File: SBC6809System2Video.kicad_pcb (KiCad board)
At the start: 4 copper layers, 161.3 x 101.9 mm, 82 parts, among them J1 DIN-9, J10 Conn_01x04, J11 Audio, J12 Conn_01x08, J13 Conn_01x08, J14 Conn_01x08, J15 Conn_01x08, J16 Conn_01x16, J17 Conn_01x08, J18 Conn_01x06, J2 Conn_Coaxial, J3 JTAG, J4 Conn_01x08, J5 Conn_01x16, J6 Conn_01x04, J7 Conn_01x08, J8 Conn_01x06, J9 Conn_01x08, U1 IDT7006L35J, U10 74LS157, U11 74LS157, U12 74LS157, U13 74LS157, U14 74LS157, U15 27C64, U16 74LS157, U2 ATF1504AS, U4 MC68B45, U5 MC68B21, U6 AD725, U7 74HCT393, U8 CD4052B, U9 GAL16V8, Y1 4.433618MHz, Y2 32MHz

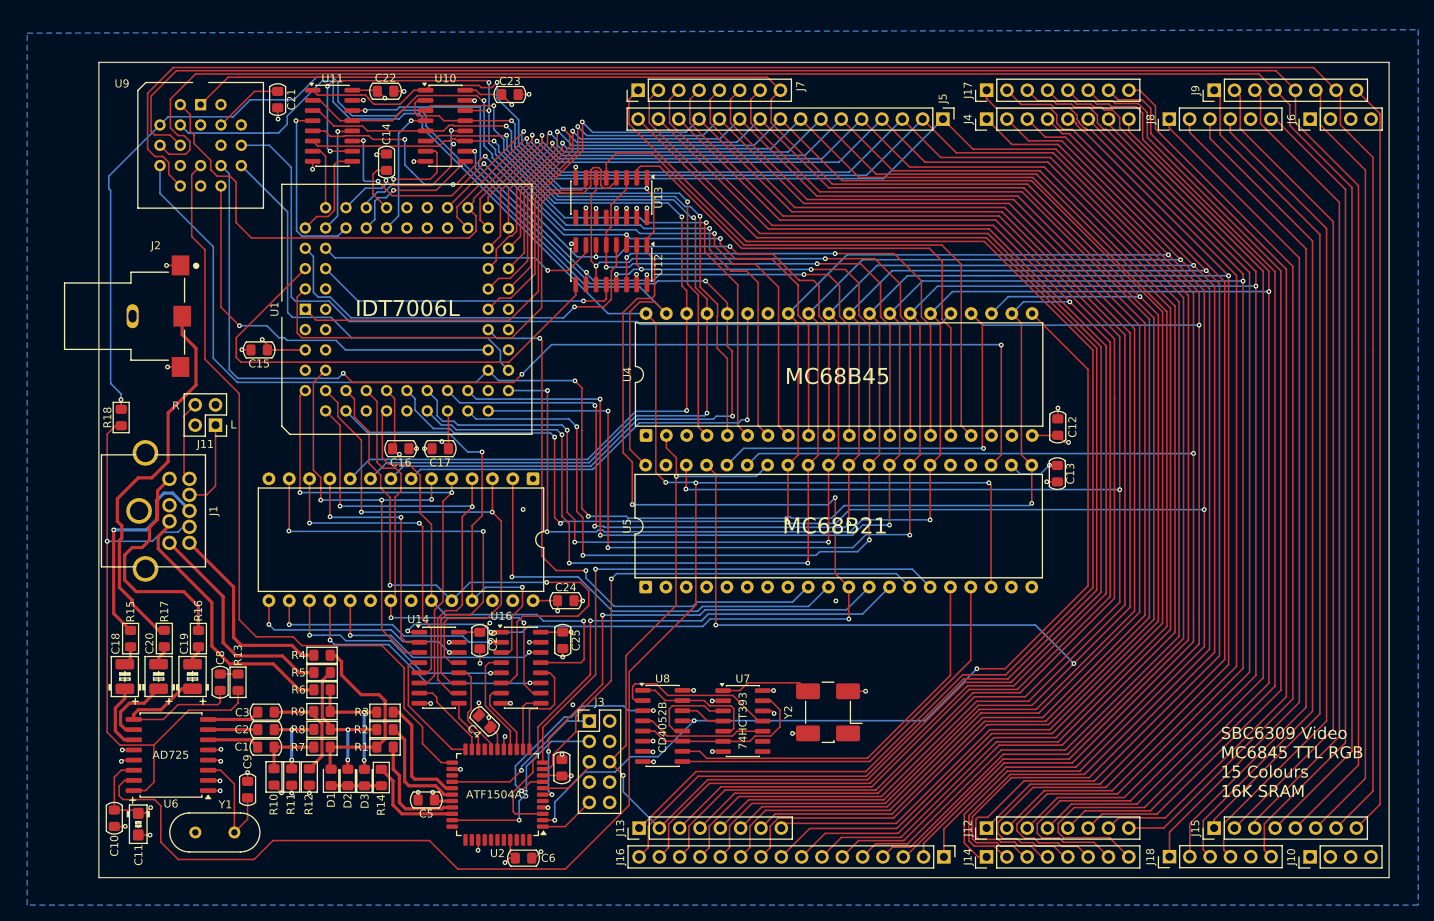
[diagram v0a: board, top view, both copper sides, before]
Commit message: convert to dragon
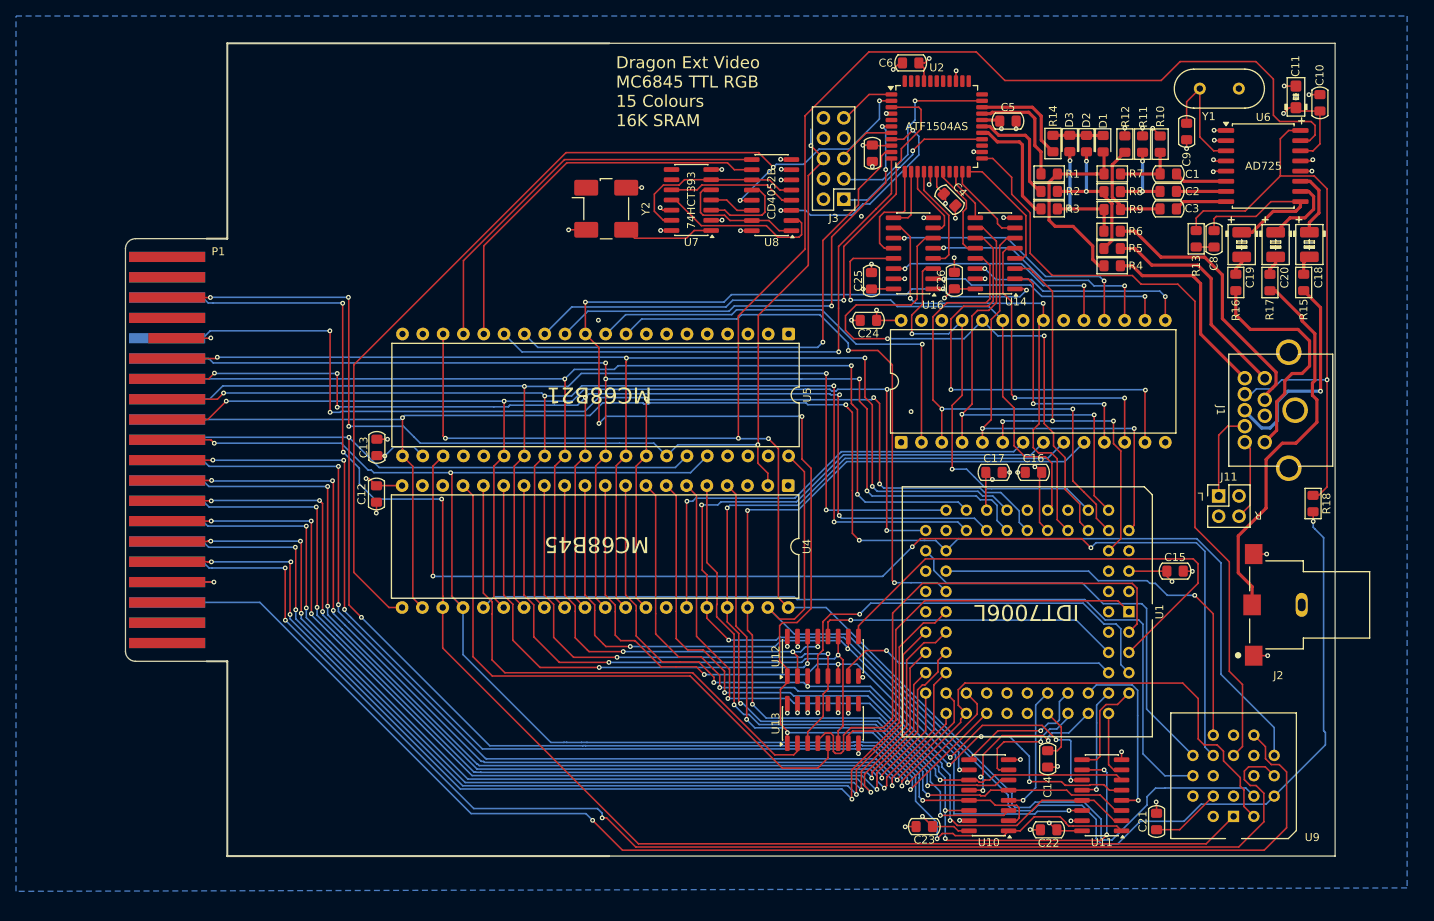
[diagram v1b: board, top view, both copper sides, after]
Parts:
- removed J10, J6: Conn_01x04, Connector_PinHeader_2.54mm:PinHeader_1x04_P2.54mm_Vertical
- removed J12, J13, J14, J15, J17, J4, J7, J9: Conn_01x08, Connector_PinHeader_2.54mm:PinHeader_1x08_P2.54mm_Vertical
- removed J16, J5: Conn_01x16, Connector_PinHeader_2.54mm:PinHeader_1x16_P2.54mm_Vertical
- removed J18, J8: Conn_01x06, Connector_PinHeader_2.54mm:PinHeader_1x06_P2.54mm_Vertical
- added P1: ~, Library:CartridgeEdge, F.Cu at (68.1, 64.9)
- moved C10 175.2 mm to (217.4, 48.2), turned to 90 degrees
- moved C11 170.9 mm to (214.4, 47.4), turned to 90 degrees
- moved Y1 160.2 mm to (207.2, 46.4), turned to 180 degrees
- moved C18 157.6 mm to (216.1, 65.9), turned to -90 degrees
- moved U9 156.8 mm to (206.6, 137.4), turned to 180 degrees
- moved U6 155.1 mm to (210.3, 56.1), turned to 0 degrees
- moved R15 153.2 mm to (215.3, 70.6), turned to -90 degrees
- moved J2 152.5 mm to (216.1, 110.9), turned to 180 degrees
- moved C20 149.7 mm to (211.8, 65.9), turned to -90 degrees
- moved R18 149.4 mm to (216.5, 98.3), turned to -90 degrees
- moved R17 145.2 mm to (211.1, 70.6), turned to -90 degrees
- moved J1 145.1 mm to (214.3, 86.6), turned to -90 degrees
- moved C9 143.3 mm to (200.7, 51.8), turned to -90 degrees
- moved C21 142.2 mm to (197.0, 138.0), turned to 90 degrees
- moved C19 141.8 mm to (207.6, 65.9), turned to -90 degrees
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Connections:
- J3 pad 10: GND -> unconnected-(J3-Pin_10-Pad10)
- J3 pad 2: GND -> unconnected-(J3-Pin_2-Pad2)
- J3 pad 4: +5V -> unconnected-(J3-Pin_4-Pad4)
- U4 pad 23: ~{E} -> E
- U9 pad 1: ~{E} -> E
- U9 pad 2: /~{SELPH} -> unconnected-(U9-I2-Pad2)
- U9 pad 6: DEV3 -> ~{R2}
- U9 pad 7: DEV4 -> unconnected-(U9-I7-Pad7)
- U9 pad 9: DEV6 -> ~{P2}
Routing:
- net DEV6: track 261.0 -> 0.00 mm
- net ~{E}: track 253.0 -> 0.00 mm, vias 1 -> 0
- net DEV4: track 252.9 -> 0.00 mm
- net DEV3: track 252.6 -> 0.00 mm
- net ~{IRQ}: track 232.1 -> 0.00 mm, vias 2 -> 0
- net ~{FIRQ}: track 224.0 -> 0.00 mm, vias 2 -> 0
- net ~{HALT}: track 174.3 -> 0.00 mm
- net A15: track 172.0 -> 0.00 mm
- net A14: track 169.9 -> 0.00 mm
- net ~{R2}: track 0.00 -> 169.5 mm, vias 0 -> 3
- net ~{P2}: track 0.00 -> 167.8 mm, vias 0 -> 1
- net A13: track 167.6 -> 0.00 mm
- net ~{NMI}: track 163.1 -> 0.00 mm
- net ~{Q}: track 161.3 -> 0.00 mm
- net D0: track 318.3 -> 159.8 mm
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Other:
- board size 161.3 x 101.9 mm -> 90.7 x 101.6 mm
- board text added: "Dragon Ext Video MC6845 TTL RGB 15 Colours 16K SRAM"
- board text removed: "SBC6309 Video MC6845 TTL RGB 15 Colours 16K SRAM"
